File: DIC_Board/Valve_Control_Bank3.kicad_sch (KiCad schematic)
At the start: 10 parts, among them U22 DRV8823QDCARQ1

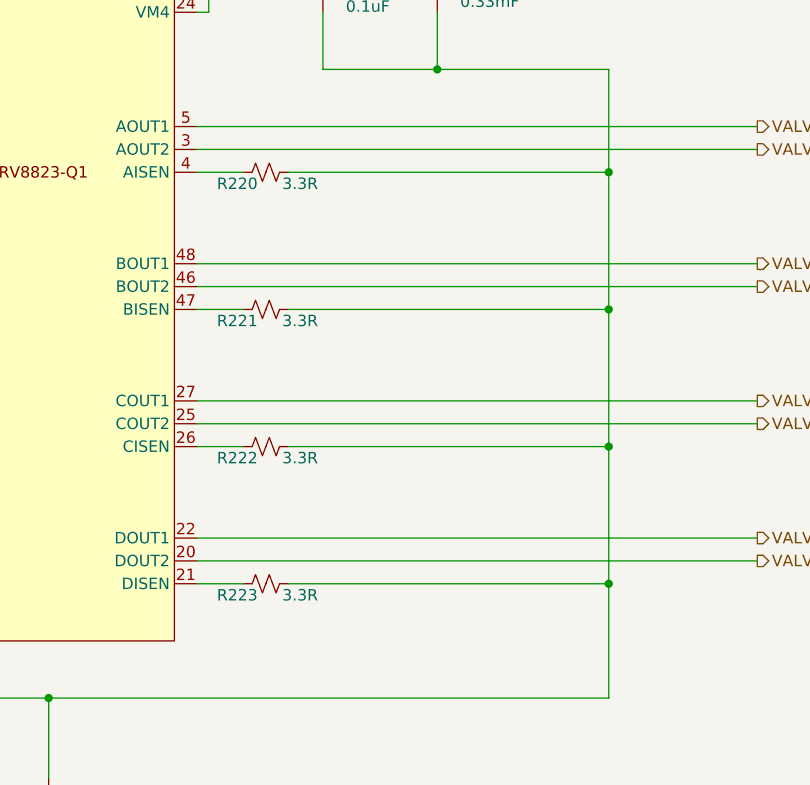
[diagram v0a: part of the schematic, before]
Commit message: Wrapping up schematic
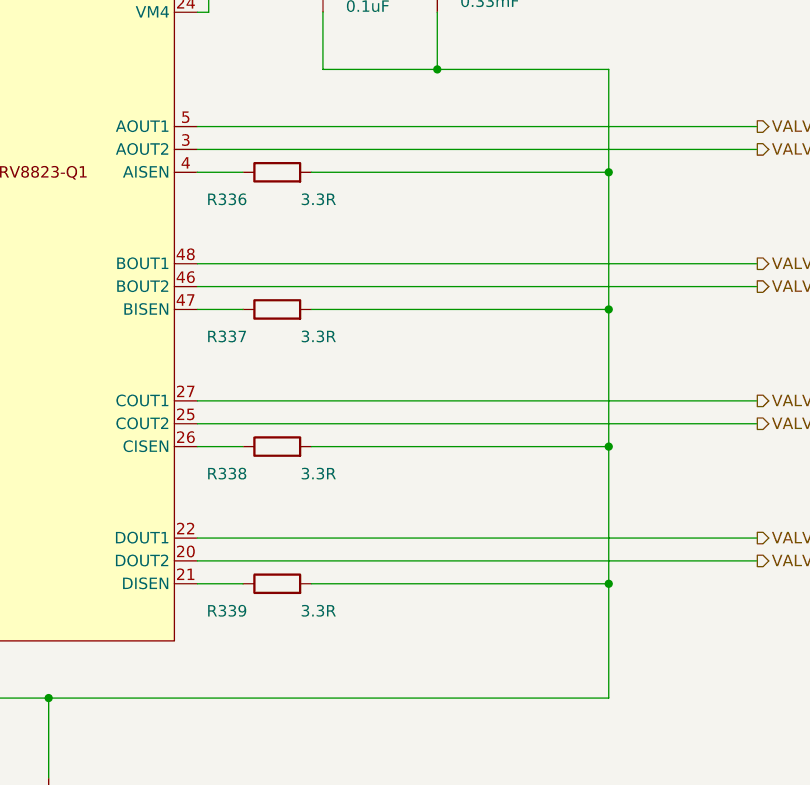
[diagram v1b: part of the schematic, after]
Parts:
- removed R220, R221, R222, R223: 3.3R, Resistor_SMD:R_1206_3216Metric, symbol Device:R_Small_US
- added R336, R337, R338, R339: 3.3R, Resistor_SMD:R_0402_1005Metric, symbol Device:R
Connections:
- net GND: now also R336.2, R337.2, R338.2, R339.2
- net at U22.26 (CISEN): now also R338.1
- net at U22.21 (DISEN): now also R339.1
- net at U22.4 (AISEN): now also R336.1
- net at U22.47 (BISEN): now also R337.1
